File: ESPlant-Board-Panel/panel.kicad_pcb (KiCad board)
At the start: 4 copper layers, 142 x 116 mm, 342 parts, among them J1 Conn_01x05, U1 HC-TYPE-C-16P-01A-G, U13 ESP32-C6-MINI-1/U, U3 AHT20-F, U5 TPS61025DRCR, U6 Light sensor, U7 TS-1088-AR02016, U8 MK-12C02-G025

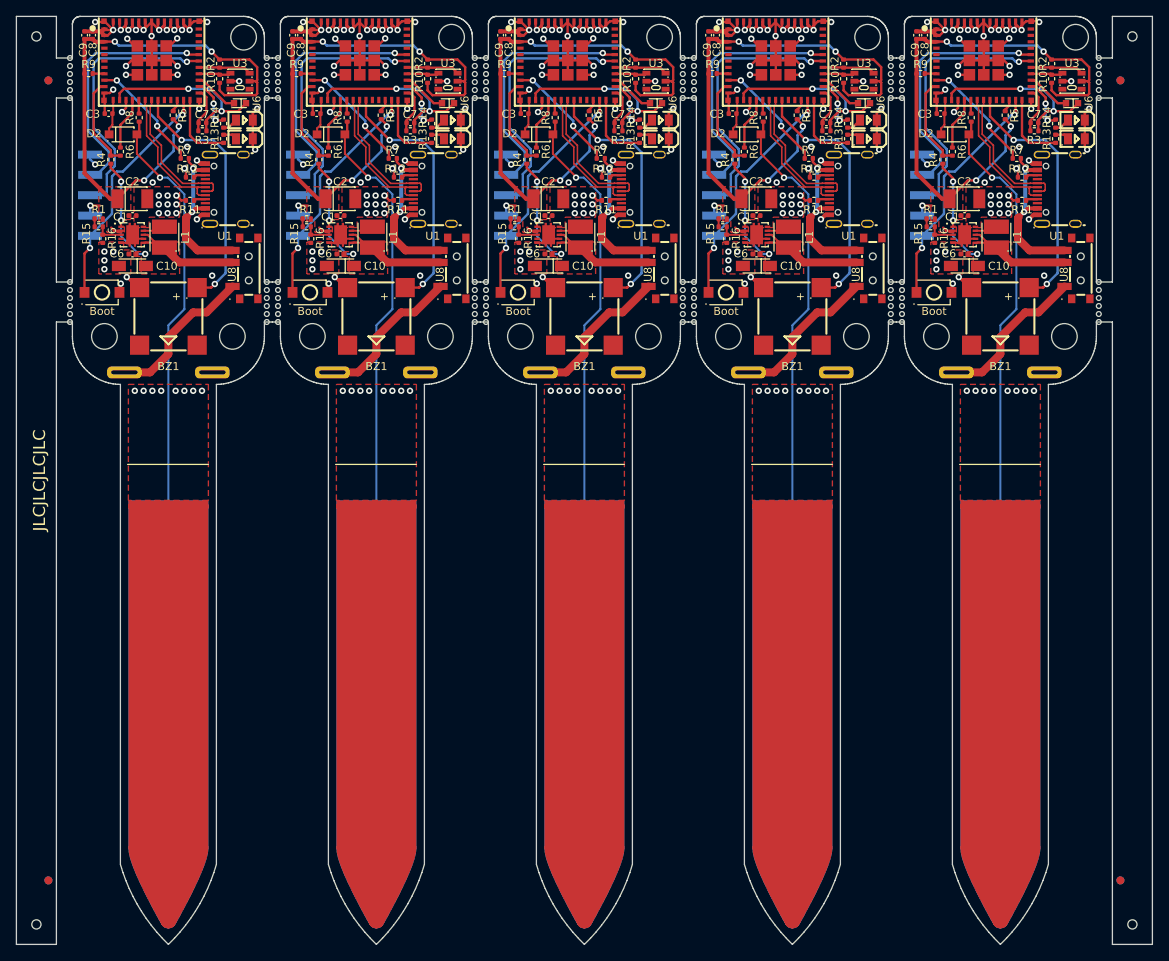
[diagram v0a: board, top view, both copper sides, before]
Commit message: Panel: Update production files
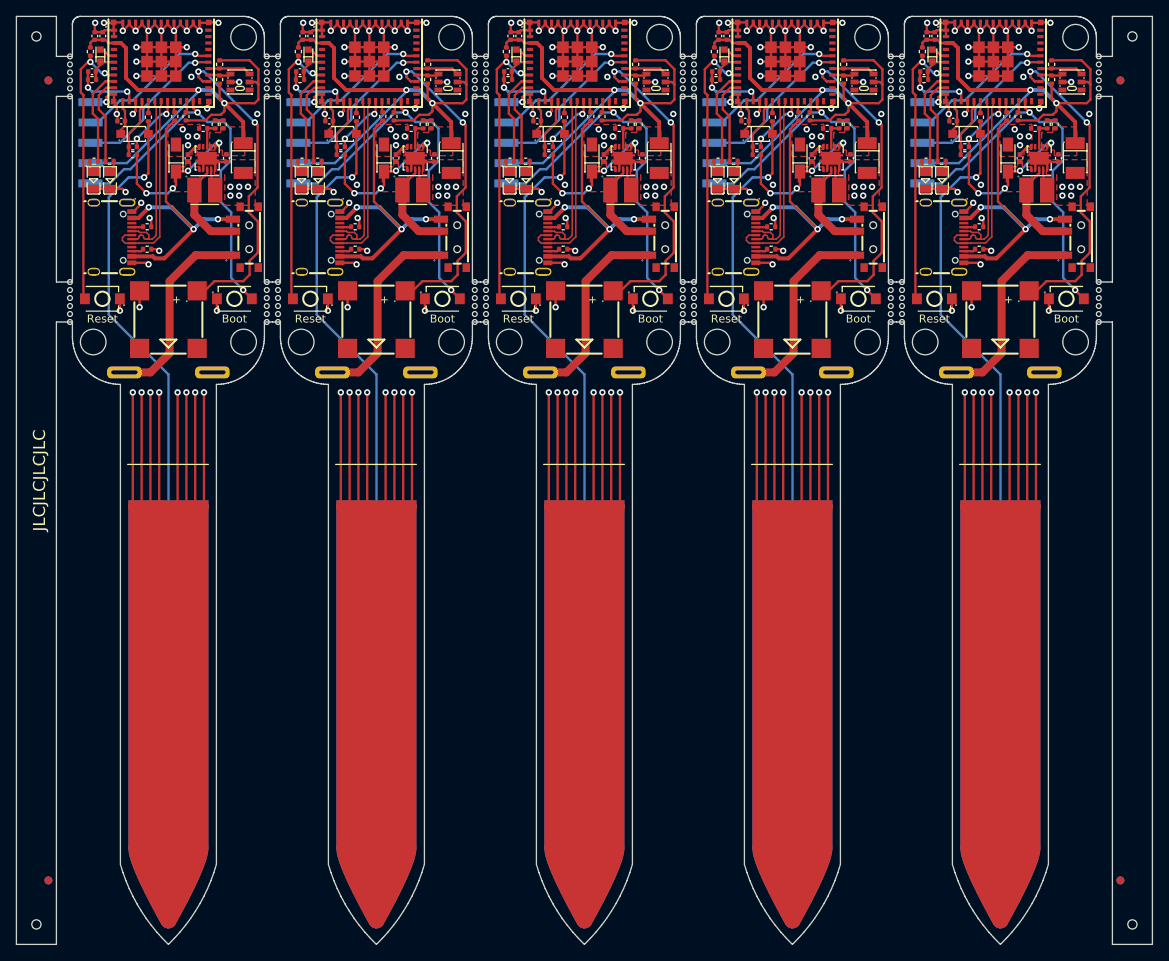
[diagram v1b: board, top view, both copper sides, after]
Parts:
- removed the BZ1 at (173.0, 57.5)
- removed the BZ1 at (251.0, 57.5)
- removed the BZ1 at (277.0, 57.5)
- removed the BZ1 at (199.0, 57.5)
- removed the BZ1 at (225.0, 57.5)
- removed the C1 at (220.5, 44.9)
- removed the C1 at (246.5, 44.9)
- removed the C1 at (194.5, 44.9)
- removed the C1 at (272.5, 44.9)
- removed the C1 at (168.5, 44.9)
- removed the C10 at (272.5, 51.2)
- removed the C10 at (194.5, 51.2)
- removed the C10 at (220.5, 51.2)
- removed the C10 at (246.5, 51.2)
- removed the C10 at (168.5, 51.2)
- removed the C2 at (168.5, 42.8)
- removed the C2 at (194.5, 42.8)
- removed the C2 at (272.5, 42.8)
- removed the C2 at (220.5, 42.8)
- removed the C2 at (246.5, 42.8)
- removed the C3 at (243.5, 32.2)
- removed the C3 at (191.5, 32.2)
- removed the C3 at (217.5, 32.2)
- removed the C3 at (165.5, 32.2)
- removed the C3 at (269.5, 32.2)
- removed the C4 at (199.0, 81.0)
- removed the C4 at (277.0, 81.0)
- removed the C4 at (173.0, 81.0)
- removed the C4 at (225.0, 81.0)
- removed the C4 at (251.0, 81.0)
- removed the C6 at (194.5, 49.7)
- removed the C6 at (246.5, 49.7)
- removed the C6 at (168.5, 49.7)
- removed the C6 at (272.5, 49.7)
- removed the C6 at (220.5, 49.7)
- removed the C7 at (255.3, 33.3)
- removed the C7 at (281.3, 33.3)
- removed the C7 at (229.3, 33.3)
- removed the C7 at (203.3, 33.3)
- removed the C7 at (177.3, 33.3)
- removed the C8 at (189.5, 22.4)
- removed the C8 at (215.5, 22.4)
- removed the C8 at (241.5, 22.4)
- removed the C8 at (267.5, 22.4)
- removed the C8 at (163.5, 22.4)
- removed the C9 at (240.5, 22.4)
- removed the C9 at (266.5, 22.4)
- removed the C9 at (162.5, 22.4)
- removed the C9 at (214.5, 22.4)
- removed the C9 at (188.5, 22.4)
- removed the D1 at (260.5, 35.3)
- removed the D1 at (208.5, 35.3)
- removed the D1 at (182.5, 35.3)
- removed the D1 at (286.5, 35.3)
- removed the D1 at (234.5, 35.3)
- removed the D2 at (219.3, 34.8)
- removed the D2 at (245.3, 34.8)
- removed the D2 at (193.3, 34.8)
- removed the D2 at (271.3, 34.8)
- removed the D2 at (167.3, 34.8)
- removed the D3 at (260.5, 33.0)
- removed the D3 at (286.5, 33.0)
- removed the D3 at (182.5, 33.0)
- removed the D3 at (234.5, 33.0)
- removed the D3 at (208.5, 33.0)
- removed the H1 at (286.4, 22.6)
- removed the H1 at (182.4, 22.6)
- removed the H1 at (260.4, 22.6)
- removed the H1 at (234.4, 22.6)
- removed the H1 at (208.4, 22.6)
- removed the H2 at (191.0, 60.0)
- removed the H2 at (243.0, 60.0)
- removed the H2 at (269.0, 60.0)
- removed the H2 at (165.0, 60.0)
- removed the H2 at (217.0, 60.0)
- removed the H3 at (259.0, 60.0)
- removed the H3 at (233.0, 60.0)
- removed the H3 at (285.0, 60.0)
- removed the H3 at (207.0, 60.0)
- removed the H3 at (181.0, 60.0)
- removed the J1 at (239.9, 42.4)
- removed the J1 at (187.9, 42.4)
- removed the J1 at (213.9, 42.4)
- removed the J1 at (265.9, 42.4)
- removed the J1 at (161.9, 42.4)
- removed the L1 at (198.5, 47.6)
- removed the L1 at (172.5, 47.6)
- removed the L1 at (250.5, 47.6)
- removed the L1 at (276.5, 47.6)
- removed the L1 at (224.5, 47.6)
- removed the R1 at (190.3, 45.3)
- removed the R1 at (164.3, 45.3)
- removed the R1 at (242.3, 45.3)
- removed the R1 at (216.3, 45.3)
- removed the R1 at (268.3, 45.3)
- removed the R10 at (283.4, 27.8)
- removed the R10 at (179.4, 27.8)
- removed the R10 at (231.4, 27.8)
- removed the R10 at (257.4, 27.8)
- removed the R10 at (205.4, 27.8)
- removed the R11 at (253.7, 43.0)
- removed the R11 at (175.7, 43.0)
- removed the R11 at (279.7, 43.0)
- removed the R11 at (227.7, 43.0)
- removed the R11 at (201.7, 43.0)
- removed the R12 at (253.7, 40.1)
- removed the R12 at (279.7, 40.1)
- removed the R12 at (175.7, 40.1)
- removed the R12 at (201.7, 40.1)
- removed the R12 at (227.7, 40.1)
- removed the R13 at (205.9, 35.3)
- removed the R13 at (231.9, 35.3)
- removed the R13 at (179.9, 35.3)
- removed the R13 at (257.9, 35.3)
- removed the R13 at (283.9, 35.3)
- removed the R14 at (179.9, 33.4)
- removed the R14 at (205.9, 33.4)
- removed the R14 at (231.9, 33.4)
- removed the R14 at (283.9, 33.4)
- removed the R14 at (257.9, 33.4)
- removed the R15 at (164.3, 46.3)
- removed the R15 at (216.3, 46.3)
- removed the R15 at (268.3, 46.3)
- removed the R15 at (242.3, 46.3)
- removed the R15 at (190.3, 46.3)
- removed the R16 at (190.8, 47.8)
- removed the R16 at (268.8, 47.8)
- removed the R16 at (216.8, 47.8)
- removed the R16 at (242.8, 47.8)
- removed the R16 at (164.8, 47.8)
- removed the R2 at (179.4, 25.9)
- removed the R2 at (283.4, 25.9)
- removed the R2 at (257.4, 25.9)
- removed the R2 at (205.4, 25.9)
- removed the R2 at (231.4, 25.9)
- removed the R3 at (203.3, 34.3)
- removed the R3 at (177.3, 34.3)
- removed the R3 at (229.3, 34.3)
- removed the R3 at (255.3, 34.3)
- removed the R3 at (281.3, 34.3)
- removed the R4 at (243.8, 37.9)
- removed the R4 at (165.8, 37.9)
- removed the R4 at (217.8, 37.9)
- removed the R4 at (191.8, 37.9)
- removed the R4 at (269.8, 37.9)
- removed the R5 at (173.6, 32.4)
- removed the R5 at (199.6, 32.4)
- removed the R5 at (251.6, 32.4)
- removed the R5 at (277.6, 32.4)
- removed the R5 at (225.6, 32.4)
- removed the R6 at (167.0, 36.9)
- removed the R6 at (193.0, 36.9)
- removed the R6 at (219.0, 36.9)
- removed the R6 at (245.0, 36.9)
- removed the R6 at (271.0, 36.9)
- removed the R7 at (227.1, 37.8)
- removed the R7 at (201.1, 37.8)
- removed the R7 at (175.1, 37.8)
- removed the R7 at (253.1, 37.8)
- removed the R7 at (279.1, 37.8)
- removed the R8 at (273.4, 32.6)
- removed the R8 at (195.4, 32.6)
- removed the R8 at (221.4, 32.6)
- removed the R8 at (247.4, 32.6)
- removed the R8 at (169.4, 32.6)
- removed the R9 at (215.0, 27.1)
- removed the R9 at (163.0, 27.1)
- removed the R9 at (267.0, 27.1)
- removed the R9 at (241.0, 27.1)
- removed the R9 at (189.0, 27.1)
- removed the U1 at (180.0, 41.6)
- removed the U1 at (232.0, 41.6)
- removed the U1 at (284.0, 41.6)
- removed the U1 at (206.0, 41.6)
- removed the U1 at (258.0, 41.6)
- removed the U13 at (274.9, 25.5)
- removed the U13 at (248.9, 25.5)
- removed the U13 at (196.9, 25.5)
- removed the U13 at (222.9, 25.5)
- removed the U13 at (170.9, 25.5)
- removed the U3 at (182.0, 28.1)
- removed the U3 at (208.0, 28.1)
- removed the U3 at (286.0, 28.1)
- removed the U3 at (234.0, 28.1)
- removed the U3 at (260.0, 28.1)
- removed the U5 at (246.5, 47.3)
- removed the U5 at (168.5, 47.3)
- removed the U5 at (272.5, 47.3)
- removed the U5 at (220.5, 47.3)
- removed the U5 at (194.5, 47.3)
- removed the U6 at (182.0, 30.9)
- removed the U6 at (234.0, 30.9)
- removed the U6 at (208.0, 30.9)
- removed the U6 at (260.0, 30.9)
- removed the U6 at (286.0, 30.9)
- removed the U7 at (242.7, 54.5)
- removed the U7 at (268.7, 54.5)
- removed the U7 at (164.7, 54.5)
- removed the U7 at (190.7, 54.5)
- removed the U7 at (216.7, 54.5)
- removed the U8 at (234.6, 51.5)
- removed the U8 at (286.6, 51.5)
- removed the U8 at (208.6, 51.5)
- removed the U8 at (182.6, 51.5)
- removed the U8 at (260.6, 51.5)
- removed the U9 at (277.0, 64.5)
- removed the U9 at (251.0, 64.5)
- removed the U9 at (173.0, 64.5)
- removed the U9 at (225.0, 64.5)
- removed the U9 at (199.0, 64.5)
- added BZ1: Buzzer, CustomFootprints:BUZ-SMD_4P-L8.5-W8.5-P8.50-BR, F.Cu at (173.0, 57.9)
- added BZ1: Buzzer, CustomFootprints:BUZ-SMD_4P-L8.5-W8.5-P8.50-BR, F.Cu at (277.0, 57.9)
- added BZ1: Buzzer, CustomFootprints:BUZ-SMD_4P-L8.5-W8.5-P8.50-BR, F.Cu at (199.0, 57.9)
- added BZ1: Buzzer, CustomFootprints:BUZ-SMD_4P-L8.5-W8.5-P8.50-BR, F.Cu at (225.0, 57.9)
- added BZ1: Buzzer, CustomFootprints:BUZ-SMD_4P-L8.5-W8.5-P8.50-BR, F.Cu at (251.0, 57.9)
- added C1: 2.2uF-Ceramic, Capacitor_SMD:C_0402_1005Metric, F.Cu at (258.3, 37.7)
- added C1: 2.2uF-Ceramic, Capacitor_SMD:C_0402_1005Metric, F.Cu at (180.3, 37.7)
- added C1: 2.2uF-Ceramic, Capacitor_SMD:C_0402_1005Metric, F.Cu at (284.3, 37.7)
- added C1: 2.2uF-Ceramic, Capacitor_SMD:C_0402_1005Metric, F.Cu at (206.3, 37.7)
- added C1: 2.2uF-Ceramic, Capacitor_SMD:C_0402_1005Metric, F.Cu at (232.3, 37.7)
- added C10: 10uF-Tantalum, CustomFootprints:CAP-SMD_L3.2-W1.6-RD-C7171, F.Cu at (200.0, 37.7)
- added C10: 10uF-Tantalum, CustomFootprints:CAP-SMD_L3.2-W1.6-RD-C7171, F.Cu at (278.0, 37.7)
- added C10: 10uF-Tantalum, CustomFootprints:CAP-SMD_L3.2-W1.6-RD-C7171, F.Cu at (252.0, 37.7)
- added C10: 10uF-Tantalum, CustomFootprints:CAP-SMD_L3.2-W1.6-RD-C7171, F.Cu at (226.0, 37.7)
- added C10: 10uF-Tantalum, CustomFootprints:CAP-SMD_L3.2-W1.6-RD-C7171, F.Cu at (174.0, 37.7)
- added C2: 100uF-Tantalum, CustomFootprints:CASE-B_3528, F.Cu at (234.4, 37.7)
- added C2: 100uF-Tantalum, CustomFootprints:CASE-B_3528, F.Cu at (208.4, 37.7)
- added C2: 100uF-Tantalum, CustomFootprints:CASE-B_3528, F.Cu at (182.4, 37.7)
- added C2: 100uF-Tantalum, CustomFootprints:CASE-B_3528, F.Cu at (260.4, 37.7)
- added C2: 100uF-Tantalum, CustomFootprints:CASE-B_3528, F.Cu at (286.4, 37.7)
- added C3: 10nF, Capacitor_SMD:C_0402_1005Metric, F.Cu at (219.1, 33.1)
- added C3: 10nF, Capacitor_SMD:C_0402_1005Metric, F.Cu at (271.1, 33.1)
- added C3: 10nF, Capacitor_SMD:C_0402_1005Metric, F.Cu at (167.1, 33.1)
- added C3: 10nF, Capacitor_SMD:C_0402_1005Metric, F.Cu at (245.1, 33.1)
- added C3: 10nF, Capacitor_SMD:C_0402_1005Metric, F.Cu at (193.1, 33.1)
- added C4: 7pF-27pF, A=2.75cm^2, CustomFootprints:Sensor-Tip, B.Cu at (251.0, 81.0)
- added C4: 7pF-27pF, A=2.75cm^2, CustomFootprints:Sensor-Tip, B.Cu at (173.0, 81.0)
- added C4: 7pF-27pF, A=2.75cm^2, CustomFootprints:Sensor-Tip, B.Cu at (277.0, 81.0)
- added C4: 7pF-27pF, A=2.75cm^2, CustomFootprints:Sensor-Tip, B.Cu at (199.0, 81.0)
- added C4: 7pF-27pF, A=2.75cm^2, CustomFootprints:Sensor-Tip, B.Cu at (225.0, 81.0)
- added C6: 100nF-Ceramic, Capacitor_SMD:C_0402_1005Metric, F.Cu at (253.5, 37.7)
- added C6: 100nF-Ceramic, Capacitor_SMD:C_0402_1005Metric, F.Cu at (279.5, 37.7)
- added C6: 100nF-Ceramic, Capacitor_SMD:C_0402_1005Metric, F.Cu at (201.5, 37.7)
- added C6: 100nF-Ceramic, Capacitor_SMD:C_0402_1005Metric, F.Cu at (175.5, 37.7)
- added C6: 100nF-Ceramic, Capacitor_SMD:C_0402_1005Metric, F.Cu at (227.5, 37.7)
- added C7: 10uF, Capacitor_SMD:C_0402_1005Metric, F.Cu at (163.5, 26.9)
- added C7: 10uF, Capacitor_SMD:C_0402_1005Metric, F.Cu at (241.5, 26.9)
- added C7: 10uF, Capacitor_SMD:C_0402_1005Metric, F.Cu at (189.5, 26.9)
- added C7: 10uF, Capacitor_SMD:C_0402_1005Metric, F.Cu at (215.5, 26.9)
- added C7: 10uF, Capacitor_SMD:C_0402_1005Metric, F.Cu at (267.5, 26.9)
- added C8: 10nF, Capacitor_SMD:C_0402_1005Metric, F.Cu at (242.8, 22.4)
- added C8: 10nF, Capacitor_SMD:C_0402_1005Metric, F.Cu at (164.8, 22.4)
- added C8: 10nF, Capacitor_SMD:C_0402_1005Metric, F.Cu at (190.8, 22.4)
- added C8: 10nF, Capacitor_SMD:C_0402_1005Metric, F.Cu at (216.8, 22.4)
- added C8: 10nF, Capacitor_SMD:C_0402_1005Metric, F.Cu at (268.8, 22.4)
- added C9: 10uF, Capacitor_SMD:C_0402_1005Metric, F.Cu at (215.8, 22.4)
- added C9: 10uF, Capacitor_SMD:C_0402_1005Metric, F.Cu at (267.8, 22.4)
- added C9: 10uF, Capacitor_SMD:C_0402_1005Metric, F.Cu at (241.8, 22.4)
- added C9: 10uF, Capacitor_SMD:C_0402_1005Metric, F.Cu at (163.8, 22.4)
- added C9: 10uF, Capacitor_SMD:C_0402_1005Metric, F.Cu at (189.8, 22.4)
- added D1: GREEN, CustomFootprints:LED0805-R-RD, F.Cu at (269.7, 40.5)
- added D1: GREEN, CustomFootprints:LED0805-R-RD, F.Cu at (191.7, 40.5)
- added D1: GREEN, CustomFootprints:LED0805-R-RD, F.Cu at (217.7, 40.5)
- added D1: GREEN, CustomFootprints:LED0805-R-RD, F.Cu at (243.7, 40.5)
- added D1: GREEN, CustomFootprints:LED0805-R-RD, F.Cu at (165.7, 40.5)
- added D2: Switching-Diode, CustomFootprints:SOD-123F_L2.7-W1.6-LS3.8-RD, F.Cu at (194.8, 34.7)
- added D2: Switching-Diode, CustomFootprints:SOD-123F_L2.7-W1.6-LS3.8-RD, F.Cu at (246.8, 34.7)
- added D2: Switching-Diode, CustomFootprints:SOD-123F_L2.7-W1.6-LS3.8-RD, F.Cu at (168.8, 34.7)
- added D2: Switching-Diode, CustomFootprints:SOD-123F_L2.7-W1.6-LS3.8-RD, F.Cu at (272.8, 34.7)
- added D2: Switching-Diode, CustomFootprints:SOD-123F_L2.7-W1.6-LS3.8-RD, F.Cu at (220.8, 34.7)
- added D3: RED, CustomFootprints:LED0805-R-RD, F.Cu at (241.7, 40.5)
- added D3: RED, CustomFootprints:LED0805-R-RD, F.Cu at (189.7, 40.5)
- added D3: RED, CustomFootprints:LED0805-R-RD, F.Cu at (215.7, 40.5)
- added D3: RED, CustomFootprints:LED0805-R-RD, F.Cu at (267.7, 40.5)
- added D3: RED, CustomFootprints:LED0805-R-RD, F.Cu at (163.7, 40.5)
- added H1: MountingHole, MountingHole:MountingHole_3.2mm_M3, F.Cu at (234.4, 22.6)
- added H1: MountingHole, MountingHole:MountingHole_3.2mm_M3, F.Cu at (286.4, 22.6)
- added H1: MountingHole, MountingHole:MountingHole_3.2mm_M3, F.Cu at (260.4, 22.6)
- added H1: MountingHole, MountingHole:MountingHole_3.2mm_M3, F.Cu at (208.4, 22.6)
- added H1: MountingHole, MountingHole:MountingHole_3.2mm_M3, F.Cu at (182.4, 22.6)
- added H2: MountingHole, MountingHole:MountingHole_3.2mm_M3, F.Cu at (241.6, 60.7)
- added H2: MountingHole, MountingHole:MountingHole_3.2mm_M3, F.Cu at (267.6, 60.7)
- added H2: MountingHole, MountingHole:MountingHole_3.2mm_M3, F.Cu at (189.6, 60.7)
- added H2: MountingHole, MountingHole:MountingHole_3.2mm_M3, F.Cu at (215.6, 60.7)
- added H2: MountingHole, MountingHole:MountingHole_3.2mm_M3, F.Cu at (163.6, 60.7)
- added H3: MountingHole, MountingHole:MountingHole_3.2mm_M3, F.Cu at (234.4, 60.7)
- added H3: MountingHole, MountingHole:MountingHole_3.2mm_M3, F.Cu at (182.4, 60.7)
- added H3: MountingHole, MountingHole:MountingHole_3.2mm_M3, F.Cu at (208.4, 60.7)
- added H3: MountingHole, MountingHole:MountingHole_3.2mm_M3, F.Cu at (260.4, 60.7)
- added H3: MountingHole, MountingHole:MountingHole_3.2mm_M3, F.Cu at (286.4, 60.7)
- added J1: Conn_01x05, CustomFootprints:PinHeader_1x05_P2.54mm_Vertical_SMD, B.Cu at (240.0, 35.8)
- added J1: Conn_01x05, CustomFootprints:PinHeader_1x05_P2.54mm_Vertical_SMD, B.Cu at (188.0, 35.8)
- added J1: Conn_01x05, CustomFootprints:PinHeader_1x05_P2.54mm_Vertical_SMD, B.Cu at (162.0, 35.8)
- added J1: Conn_01x05, CustomFootprints:PinHeader_1x05_P2.54mm_Vertical_SMD, B.Cu at (266.0, 35.8)
- added J1: Conn_01x05, CustomFootprints:PinHeader_1x05_P2.54mm_Vertical_SMD, B.Cu at (214.0, 35.8)
- added L1: 6.8uH, CustomFootprints:IND-SMD_L3.5-W3.0, F.Cu at (281.6, 41.7)
- added L1: 6.8uH, CustomFootprints:IND-SMD_L3.5-W3.0, F.Cu at (255.6, 41.7)
- added L1: 6.8uH, CustomFootprints:IND-SMD_L3.5-W3.0, F.Cu at (177.6, 41.7)
- added L1: 6.8uH, CustomFootprints:IND-SMD_L3.5-W3.0, F.Cu at (229.6, 41.7)
- added L1: 6.8uH, CustomFootprints:IND-SMD_L3.5-W3.0, F.Cu at (203.6, 41.7)
- added R1: 100k, Resistor_SMD:R_0402_1005Metric, F.Cu at (205.9, 33.5)
- added R1: 100k, Resistor_SMD:R_0402_1005Metric, F.Cu at (257.9, 33.5)
- added R1: 100k, Resistor_SMD:R_0402_1005Metric, F.Cu at (179.9, 33.5)
- added R1: 100k, Resistor_SMD:R_0402_1005Metric, F.Cu at (231.9, 33.5)
- added R1: 100k, Resistor_SMD:R_0402_1005Metric, F.Cu at (283.9, 33.5)
- added R10: 5k1, Resistor_SMD:R_0402_1005Metric, F.Cu at (179.4, 27.9)
- added R10: 5k1, Resistor_SMD:R_0402_1005Metric, F.Cu at (283.4, 27.9)
- added R10: 5k1, Resistor_SMD:R_0402_1005Metric, F.Cu at (205.4, 27.9)
- added R10: 5k1, Resistor_SMD:R_0402_1005Metric, F.Cu at (231.4, 27.9)
- added R10: 5k1, Resistor_SMD:R_0402_1005Metric, F.Cu at (257.4, 27.9)
- added R11: 5k1, Resistor_SMD:R_0402_1005Metric, F.Cu at (248.4, 46.3)
- added R11: 5k1, Resistor_SMD:R_0402_1005Metric, F.Cu at (196.4, 46.3)
- added R11: 5k1, Resistor_SMD:R_0402_1005Metric, F.Cu at (170.4, 46.3)
- added R11: 5k1, Resistor_SMD:R_0402_1005Metric, F.Cu at (222.4, 46.3)
- added R11: 5k1, Resistor_SMD:R_0402_1005Metric, F.Cu at (274.4, 46.3)
- added R12: 5k1, Resistor_SMD:R_0402_1005Metric, F.Cu at (196.4, 49.1)
- added R12: 5k1, Resistor_SMD:R_0402_1005Metric, F.Cu at (274.4, 49.1)
- added R12: 5k1, Resistor_SMD:R_0402_1005Metric, F.Cu at (170.4, 49.1)
- added R12: 5k1, Resistor_SMD:R_0402_1005Metric, F.Cu at (222.4, 49.1)
- added R12: 5k1, Resistor_SMD:R_0402_1005Metric, F.Cu at (248.4, 49.1)
- added R13: 120, Resistor_SMD:R_0402_1005Metric, F.Cu at (165.7, 38.1)
- added R13: 120, Resistor_SMD:R_0402_1005Metric, F.Cu at (269.7, 38.1)
- added R13: 120, Resistor_SMD:R_0402_1005Metric, F.Cu at (243.7, 38.1)
- added R13: 120, Resistor_SMD:R_0402_1005Metric, F.Cu at (191.7, 38.1)
- added R13: 120, Resistor_SMD:R_0402_1005Metric, F.Cu at (217.7, 38.1)
- added R14: 120, Resistor_SMD:R_0402_1005Metric, F.Cu at (215.7, 38.1)
- added R14: 120, Resistor_SMD:R_0402_1005Metric, F.Cu at (241.7, 38.1)
- added R14: 120, Resistor_SMD:R_0402_1005Metric, F.Cu at (163.7, 38.1)
- added R14: 120, Resistor_SMD:R_0402_1005Metric, F.Cu at (189.7, 38.1)
- added R14: 120, Resistor_SMD:R_0402_1005Metric, F.Cu at (267.7, 38.1)
- added R15: 1M, Resistor_SMD:R_0402_1005Metric, F.Cu at (178.9, 33.5)
- added R15: 1M, Resistor_SMD:R_0402_1005Metric, F.Cu at (230.9, 33.5)
- added R15: 1M, Resistor_SMD:R_0402_1005Metric, F.Cu at (204.9, 33.5)
- added R15: 1M, Resistor_SMD:R_0402_1005Metric, F.Cu at (282.9, 33.5)
- added R15: 1M, Resistor_SMD:R_0402_1005Metric, F.Cu at (256.9, 33.5)
- added R16: 200k, Resistor_SMD:R_0402_1005Metric, F.Cu at (203.4, 34.0)
- added R16: 200k, Resistor_SMD:R_0402_1005Metric, F.Cu at (229.4, 34.0)
- added R16: 200k, Resistor_SMD:R_0402_1005Metric, F.Cu at (177.4, 34.0)
- added R16: 200k, Resistor_SMD:R_0402_1005Metric, F.Cu at (281.4, 34.0)
- added R16: 200k, Resistor_SMD:R_0402_1005Metric, F.Cu at (255.4, 34.0)
- added R2: 5k1, Resistor_SMD:R_0402_1005Metric, F.Cu at (179.4, 26.0)
- added R2: 5k1, Resistor_SMD:R_0402_1005Metric, F.Cu at (205.4, 26.0)
- added R2: 5k1, Resistor_SMD:R_0402_1005Metric, F.Cu at (283.4, 26.0)
- added R2: 5k1, Resistor_SMD:R_0402_1005Metric, F.Cu at (257.4, 26.0)
- added R2: 5k1, Resistor_SMD:R_0402_1005Metric, F.Cu at (231.4, 26.0)
- added R3: 47k, Resistor_SMD:R_0402_1005Metric, F.Cu at (267.5, 27.9)
- added R3: 47k, Resistor_SMD:R_0402_1005Metric, F.Cu at (241.5, 27.9)
- added R3: 47k, Resistor_SMD:R_0402_1005Metric, F.Cu at (215.5, 27.9)
- added R3: 47k, Resistor_SMD:R_0402_1005Metric, F.Cu at (163.5, 27.9)
- added R3: 47k, Resistor_SMD:R_0402_1005Metric, F.Cu at (189.5, 27.9)
- added R4: 5k1, Resistor_SMD:R_0402_1005Metric, F.Cu at (246.6, 37.3)
- added R4: 5k1, Resistor_SMD:R_0402_1005Metric, F.Cu at (194.6, 37.3)
- added R4: 5k1, Resistor_SMD:R_0402_1005Metric, F.Cu at (168.6, 37.3)
- added R4: 5k1, Resistor_SMD:R_0402_1005Metric, F.Cu at (220.6, 37.3)
- added R4: 5k1, Resistor_SMD:R_0402_1005Metric, F.Cu at (272.6, 37.3)
- added R5: 10k, Resistor_SMD:R_0402_1005Metric, F.Cu at (253.2, 32.5)
- added R5: 10k, Resistor_SMD:R_0402_1005Metric, F.Cu at (201.2, 32.5)
- added R5: 10k, Resistor_SMD:R_0402_1005Metric, F.Cu at (227.2, 32.5)
- added R5: 10k, Resistor_SMD:R_0402_1005Metric, F.Cu at (175.2, 32.5)
- added R5: 10k, Resistor_SMD:R_0402_1005Metric, F.Cu at (279.2, 32.5)
- added R6: 2k, Resistor_SMD:R_0402_1005Metric, F.Cu at (272.6, 36.3)
- added R6: 2k, Resistor_SMD:R_0402_1005Metric, F.Cu at (194.6, 36.3)
- added R6: 2k, Resistor_SMD:R_0402_1005Metric, F.Cu at (246.6, 36.3)
- added R6: 2k, Resistor_SMD:R_0402_1005Metric, F.Cu at (168.6, 36.3)
- added R6: 2k, Resistor_SMD:R_0402_1005Metric, F.Cu at (220.6, 36.3)
- added R7: 10k, Resistor_SMD:R_0402_1005Metric, F.Cu at (225.8, 32.5)
- added R7: 10k, Resistor_SMD:R_0402_1005Metric, F.Cu at (199.8, 32.5)
- added R7: 10k, Resistor_SMD:R_0402_1005Metric, F.Cu at (173.8, 32.5)
- added R7: 10k, Resistor_SMD:R_0402_1005Metric, F.Cu at (251.8, 32.5)
- added R7: 10k, Resistor_SMD:R_0402_1005Metric, F.Cu at (277.8, 32.5)
- added R8: 10k, Resistor_SMD:R_0402_1005Metric, F.Cu at (170.5, 32.6)
- added R8: 10k, Resistor_SMD:R_0402_1005Metric, F.Cu at (196.5, 32.6)
- added R8: 10k, Resistor_SMD:R_0402_1005Metric, F.Cu at (248.5, 32.6)
- added R8: 10k, Resistor_SMD:R_0402_1005Metric, F.Cu at (222.5, 32.6)
- added R8: 10k, Resistor_SMD:R_0402_1005Metric, F.Cu at (274.5, 32.6)
- added R9: 10k, Resistor_SMD:R_0402_1005Metric, F.Cu at (267.3, 24.4)
- added R9: 10k, Resistor_SMD:R_0402_1005Metric, F.Cu at (189.3, 24.4)
- added R9: 10k, Resistor_SMD:R_0402_1005Metric, F.Cu at (163.3, 24.4)
- added R9: 10k, Resistor_SMD:R_0402_1005Metric, F.Cu at (215.3, 24.4)
- added R9: 10k, Resistor_SMD:R_0402_1005Metric, F.Cu at (241.3, 24.4)
- added U1: USB-C, CustomFootprints:USB-C-SMD_G-SWITCH_GT-USB-7010EN, F.Cu at (166.1, 47.6)
- added U1: USB-C, CustomFootprints:USB-C-SMD_G-SWITCH_GT-USB-7010EN, F.Cu at (192.1, 47.6)
- added U1: USB-C, CustomFootprints:USB-C-SMD_G-SWITCH_GT-USB-7010EN, F.Cu at (218.1, 47.6)
- added U1: USB-C, CustomFootprints:USB-C-SMD_G-SWITCH_GT-USB-7010EN, F.Cu at (270.1, 47.6)
- added U1: USB-C, CustomFootprints:USB-C-SMD_G-SWITCH_GT-USB-7010EN, F.Cu at (244.1, 47.6)
- added U13: ESP32-C6-MINI-1-N4, CustomFootprints:WIFIM-SMD_61P-L16.6-W13.2-P0.80-ESP32-C6-MINI-1-N4, F.Cu at (276.1, 25.7)
- added U13: ESP32-C6-MINI-1-N4, CustomFootprints:WIFIM-SMD_61P-L16.6-W13.2-P0.80-ESP32-C6-MINI-1-N4, F.Cu at (250.1, 25.7)
- added U13: ESP32-C6-MINI-1-N4, CustomFootprints:WIFIM-SMD_61P-L16.6-W13.2-P0.80-ESP32-C6-MINI-1-N4, F.Cu at (224.1, 25.7)
- added U13: ESP32-C6-MINI-1-N4, CustomFootprints:WIFIM-SMD_61P-L16.6-W13.2-P0.80-ESP32-C6-MINI-1-N4, F.Cu at (198.1, 25.7)
- added U13: ESP32-C6-MINI-1-N4, CustomFootprints:WIFIM-SMD_61P-L16.6-W13.2-P0.80-ESP32-C6-MINI-1-N4, F.Cu at (172.1, 25.7)
- added U3: AHT20-F, CustomFootprints:SENSOR-SMD-6_AHT20, F.Cu at (208.0, 28.2)
- added U3: AHT20-F, CustomFootprints:SENSOR-SMD-6_AHT20, F.Cu at (234.0, 28.2)
- added U3: AHT20-F, CustomFootprints:SENSOR-SMD-6_AHT20, F.Cu at (260.0, 28.2)
- added U3: AHT20-F, CustomFootprints:SENSOR-SMD-6_AHT20, F.Cu at (286.0, 28.2)
- added U3: AHT20-F, CustomFootprints:SENSOR-SMD-6_AHT20, F.Cu at (182.0, 28.2)
- added U4: Tactile-Switch, CustomFootprints:SW-SMD_L3.9-W3.0-P4.45, F.Cu at (216.8, 55.3)
- added U4: Tactile-Switch, CustomFootprints:SW-SMD_L3.9-W3.0-P4.45, F.Cu at (242.8, 55.3)
- added U4: Tactile-Switch, CustomFootprints:SW-SMD_L3.9-W3.0-P4.45, F.Cu at (268.8, 55.3)
- added U4: Tactile-Switch, CustomFootprints:SW-SMD_L3.9-W3.0-P4.45, F.Cu at (164.8, 55.3)
- added U4: Tactile-Switch, CustomFootprints:SW-SMD_L3.9-W3.0-P4.45, F.Cu at (190.8, 55.3)
- added U5: 3.3V-Regulator, CustomFootprints:VSON-10_L3.0-W3.0-P0.50-BL-EP_TPS62410DRCR, F.Cu at (255.9, 37.7)
- added U5: 3.3V-Regulator, CustomFootprints:VSON-10_L3.0-W3.0-P0.50-BL-EP_TPS62410DRCR, F.Cu at (281.9, 37.7)
- added U5: 3.3V-Regulator, CustomFootprints:VSON-10_L3.0-W3.0-P0.50-BL-EP_TPS62410DRCR, F.Cu at (177.9, 37.7)
- added U5: 3.3V-Regulator, CustomFootprints:VSON-10_L3.0-W3.0-P0.50-BL-EP_TPS62410DRCR, F.Cu at (229.9, 37.7)
- added U5: 3.3V-Regulator, CustomFootprints:VSON-10_L3.0-W3.0-P0.50-BL-EP_TPS62410DRCR, F.Cu at (203.9, 37.7)
- added U6: Light sensor, CustomFootprints:SENSORS-SMD_ALS-PT19, F.Cu at (216.5, 24.9)
- added U6: Light sensor, CustomFootprints:SENSORS-SMD_ALS-PT19, F.Cu at (190.5, 24.9)
- added U6: Light sensor, CustomFootprints:SENSORS-SMD_ALS-PT19, F.Cu at (242.5, 24.9)
- added U6: Light sensor, CustomFootprints:SENSORS-SMD_ALS-PT19, F.Cu at (164.5, 24.9)
- added U6: Light sensor, CustomFootprints:SENSORS-SMD_ALS-PT19, F.Cu at (268.5, 24.9)
- added U7: Tactile-Switch, CustomFootprints:SW-SMD_L3.9-W3.0-P4.45, F.Cu at (259.3, 55.3)
- added U7: Tactile-Switch, CustomFootprints:SW-SMD_L3.9-W3.0-P4.45, F.Cu at (207.3, 55.3)
- added U7: Tactile-Switch, CustomFootprints:SW-SMD_L3.9-W3.0-P4.45, F.Cu at (181.3, 55.3)
- added U7: Tactile-Switch, CustomFootprints:SW-SMD_L3.9-W3.0-P4.45, F.Cu at (233.3, 55.3)
- added U7: Tactile-Switch, CustomFootprints:SW-SMD_L3.9-W3.0-P4.45, F.Cu at (285.3, 55.3)
- added U8: Slide-Switch, CustomFootprints:SW-SMD_MK-12C02-G025, F.Cu at (234.7, 47.6)
- added U8: Slide-Switch, CustomFootprints:SW-SMD_MK-12C02-G025, F.Cu at (260.7, 47.6)
- added U8: Slide-Switch, CustomFootprints:SW-SMD_MK-12C02-G025, F.Cu at (182.7, 47.6)
- added U8: Slide-Switch, CustomFootprints:SW-SMD_MK-12C02-G025, F.Cu at (208.7, 47.6)
- added U8: Slide-Switch, CustomFootprints:SW-SMD_MK-12C02-G025, F.Cu at (286.7, 47.6)
- added U9: Battery-Spring, CustomFootprints:AAA Battery-spring, B.Cu at (277.0, 64.5)
- added U9: Battery-Spring, CustomFootprints:AAA Battery-spring, B.Cu at (199.0, 64.5)
- added U9: Battery-Spring, CustomFootprints:AAA Battery-spring, B.Cu at (225.0, 64.5)
- added U9: Battery-Spring, CustomFootprints:AAA Battery-spring, B.Cu at (251.0, 64.5)
- added U9: Battery-Spring, CustomFootprints:AAA Battery-spring, B.Cu at (173.0, 64.5)
- moved KiKit_MB_12_1 0.20 mm to (212.7, 25.0)
- moved KiKit_MB_12_2 0.20 mm to (212.7, 26.0)
- moved KiKit_MB_12_3 0.20 mm to (212.7, 27.0)
- moved KiKit_MB_12_4 0.20 mm to (212.7, 28.0)
- moved KiKit_MB_12_5 0.20 mm to (212.7, 29.0)
- moved KiKit_MB_12_6 0.20 mm to (212.7, 30.0)
- moved KiKit_MB_16_1 0.20 mm to (238.7, 25.0)
- moved KiKit_MB_16_2 0.20 mm to (238.7, 26.0)
- moved KiKit_MB_16_3 0.20 mm to (238.7, 27.0)
- moved KiKit_MB_16_4 0.20 mm to (238.7, 28.0)
- moved KiKit_MB_16_5 0.20 mm to (238.7, 29.0)
- moved KiKit_MB_16_6 0.20 mm to (238.7, 30.0)
- moved KiKit_MB_20_1 0.20 mm to (264.7, 25.0)
- moved KiKit_MB_20_2 0.20 mm to (264.7, 26.0)
- moved KiKit_MB_20_3 0.20 mm to (264.7, 27.0)
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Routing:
- net Board_2-GND: track 84.1 -> 214.8 mm, vias 55 -> 47
- net Board_0-GND: track 84.1 -> 214.8 mm, vias 55 -> 47
- net Board_4-GND: track 84.1 -> 214.8 mm, vias 55 -> 47
- net Board_3-GND: track 84.1 -> 214.8 mm, vias 55 -> 47
- net Board_1-GND: track 84.1 -> 214.8 mm, vias 55 -> 47
- net Board_3-Moisture_SensorCapV: track 0.00 -> 54.2 mm, vias 0 -> 1
- net Board_2-Moisture_SensorCapV: track 0.00 -> 54.2 mm, vias 0 -> 1
- net Board_1-Moisture_SensorCapV: track 0.00 -> 54.2 mm, vias 0 -> 1
- net Board_0-Moisture_SensorCapV: track 0.00 -> 54.2 mm, vias 0 -> 1
- net Board_4-Moisture_SensorCapV: track 0.00 -> 54.2 mm, vias 0 -> 1
- net Board_3-/SensorCapV: track 51.8 -> 0.00 mm, vias 1 -> 0
- net Board_2-/SensorCapV: track 51.8 -> 0.00 mm, vias 1 -> 0
- net Board_1-/SensorCapV: track 51.8 -> 0.00 mm, vias 1 -> 0
- net Board_0-/SensorCapV: track 51.8 -> 0.00 mm, vias 1 -> 0
- net Board_4-/SensorCapV: track 51.8 -> 0.00 mm, vias 1 -> 0
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- added copper zone on F.Cu, net Board_0-PWR_VIN
- added copper zone on F.Cu, net Board_1-PWR_VIN
- added copper zone on F.Cu, net Board_2-PWR_VIN
- added copper zone on F.Cu, net Board_3-PWR_VIN
- added copper zone on F.Cu, net Board_4-PWR_VIN
- removed copper zone on F.Cu, net Board_0-VCC
- removed copper zone on F.Cu, net Board_1-VCC
- removed copper zone on F.Cu, net Board_2-VCC
- removed copper zone on F.Cu, net Board_3-VCC
- removed copper zone on F.Cu, net Board_4-VCC
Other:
- outline, holes or cut-outs redrawn
- board text added: "Reset"
- board text added: "USB〡BAT"
